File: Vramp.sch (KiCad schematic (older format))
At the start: 11 parts

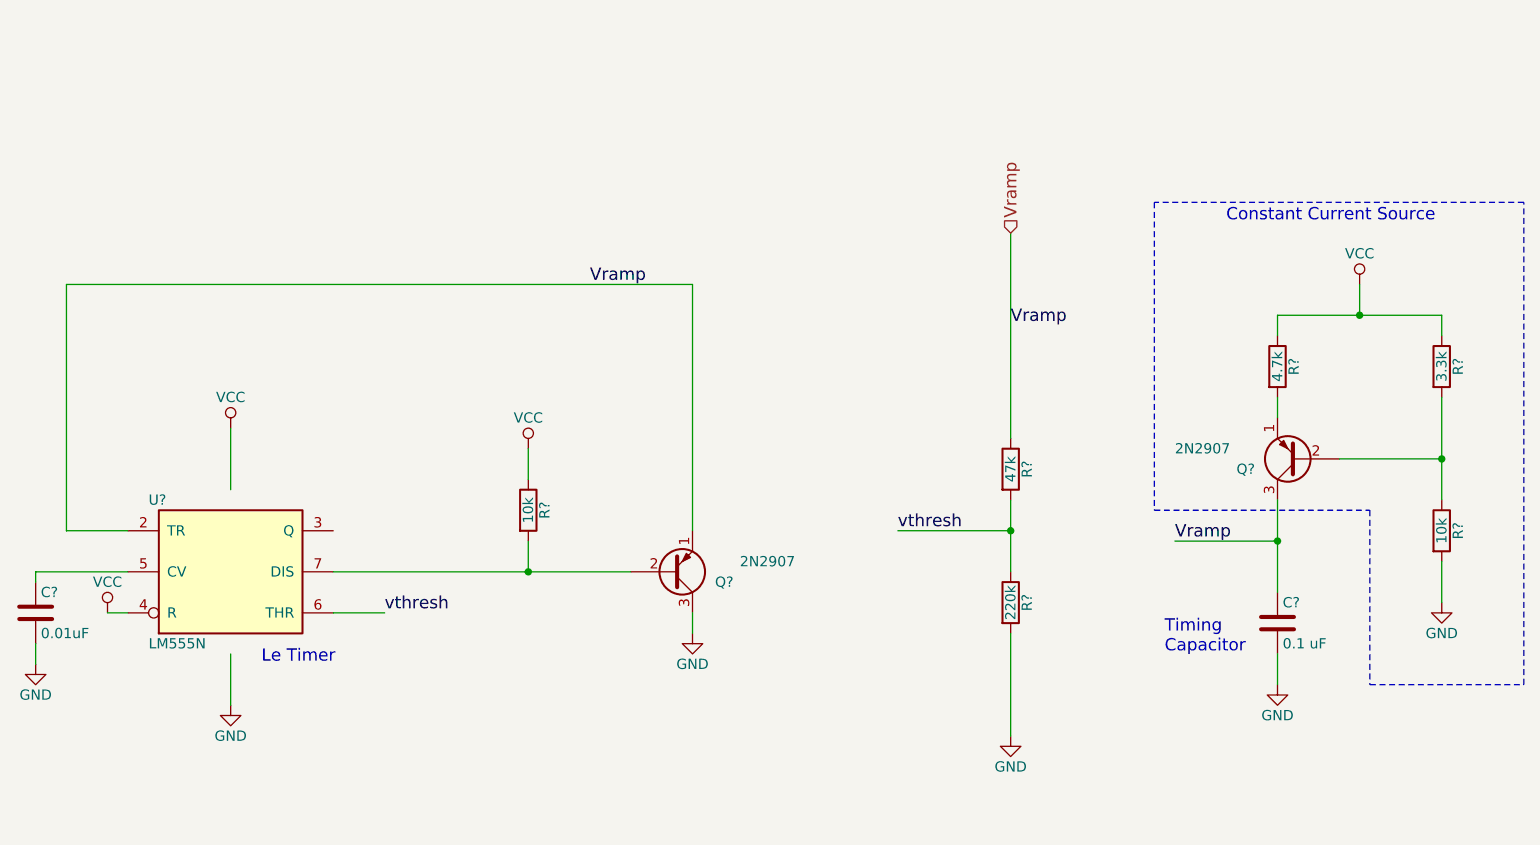
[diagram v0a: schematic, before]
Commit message: Added some text to make things more obvious
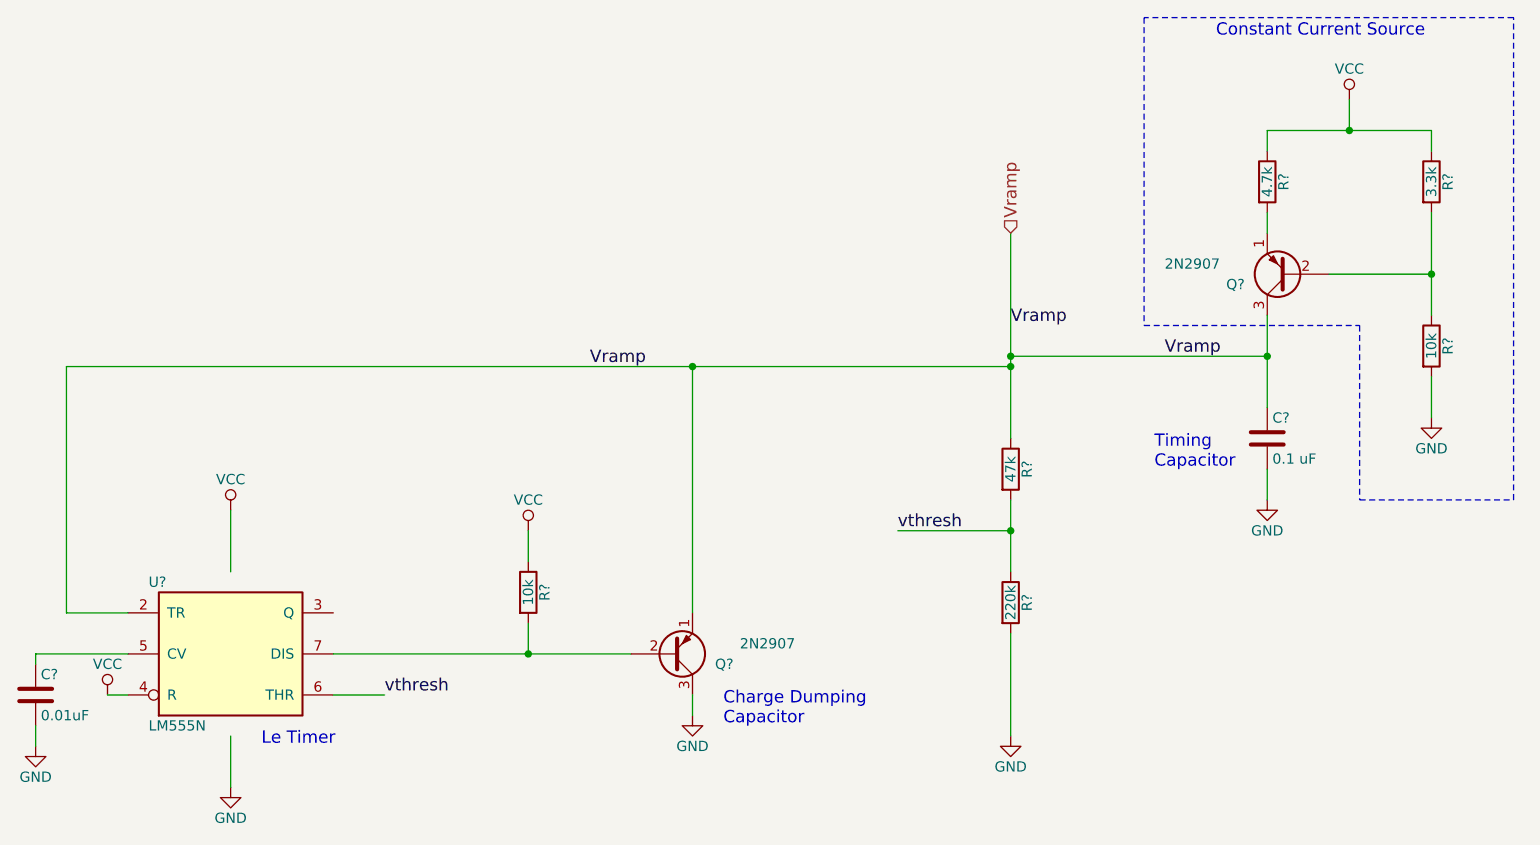
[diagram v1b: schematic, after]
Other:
- note added: "Charge Dumping\nCapacitor"
- moved on the sheet: C?, Q?, R?, U?
